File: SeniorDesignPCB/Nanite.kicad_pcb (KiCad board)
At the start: 2 copper layers, 154.9 x 76.2 mm, 20 parts, among them U1 4017, U2 TLC555

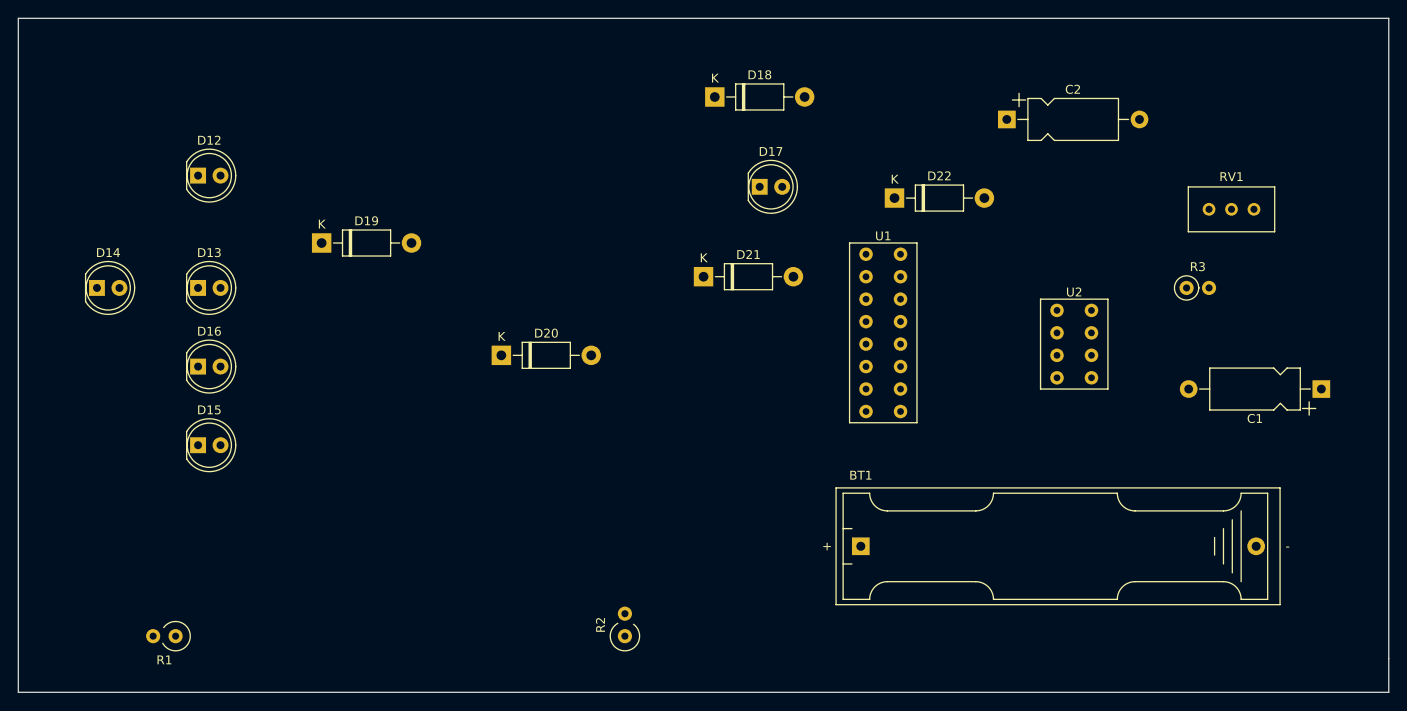
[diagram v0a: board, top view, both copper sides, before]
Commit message: Added all tracings
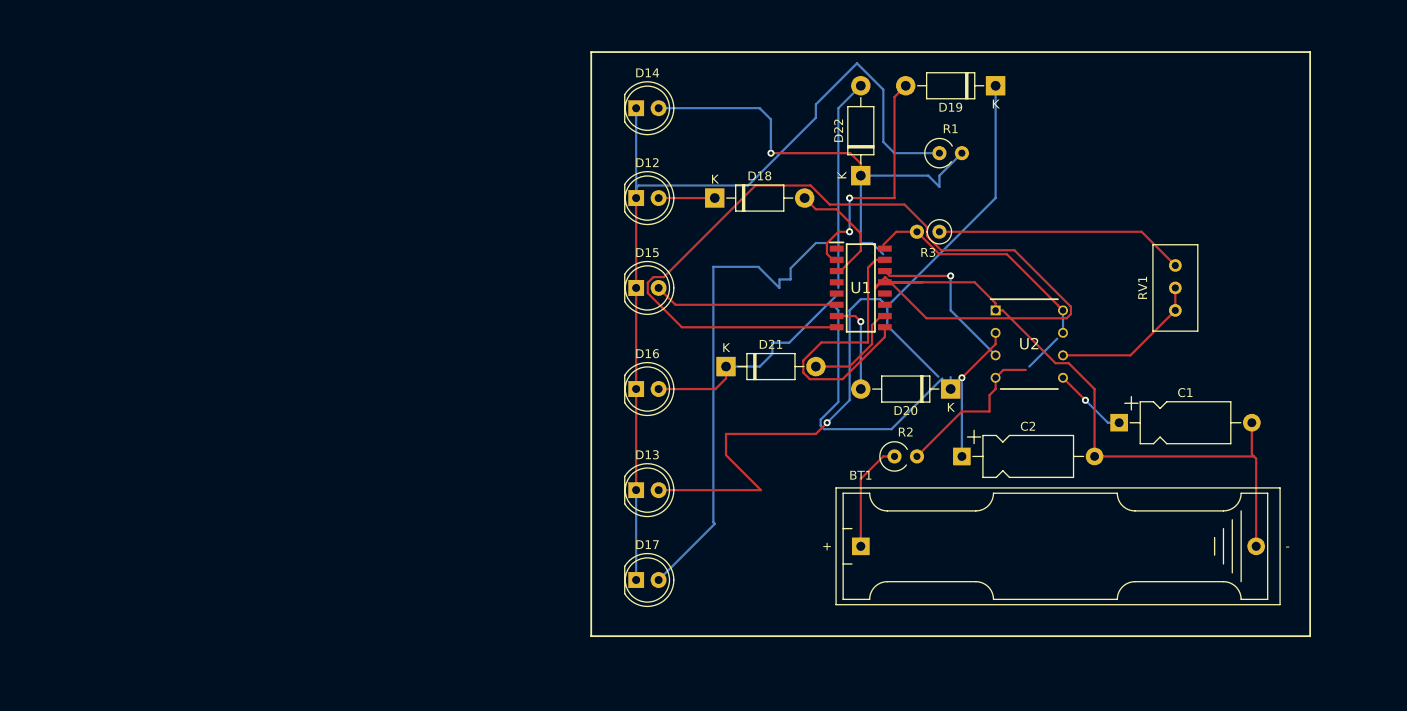
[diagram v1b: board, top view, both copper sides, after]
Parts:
- U1: footprint Johnson Counter 4017:DecadeCounter -> 74HC4017D_653:SOIC127P600X175-16N
- U2: value TLC555 -> 555TIMER; footprint 555 Timer:TLC555 -> LM555CN_Timer:DIP762W53P254L980H533Q8N
- moved R1 102.2 mm to (127.0, 77.5), turned to 0 degrees
- moved D19 78.2 mm to (133.3, 69.8), turned to 180 degrees
- moved D14 64.3 mm to (92.7, 72.4)
- moved D13 54.6 mm to (92.7, 115.6)
- moved D15 52.6 mm to (92.7, 92.7)
- moved D20 50.9 mm to (128.3, 104.1), turned to 180 degrees
- moved D12 49.6 mm to (92.7, 82.5)
- moved D16 49.6 mm to (92.7, 104.1)
- moved D17 46.6 mm to (92.7, 125.7)
- moved C2 38.4 mm to (129.5, 111.8)
- moved R2 36.6 mm to (121.9, 111.8), turned to 0 degrees
- moved R3 28.7 mm to (127.0, 86.4), turned to 180 degrees
- moved C1 23.2 mm to (147.3, 108.0), turned to 0 degrees
- moved D18 11.4 mm to (101.6, 82.5)
- moved RV1 10.9 mm to (153.7, 90.2), turned to 90 degrees
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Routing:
- net GNDA: track 0.00 -> 186.4 mm
- net Net-(D12-Pad1): track 0.00 -> 103.2 mm
- net Net-(D13-Pad2): track 0.00 -> 90.8 mm, vias 0 -> 1
- net Net-(D14-Pad2): track 0.00 -> 86.9 mm, vias 0 -> 1
- net Net-(D17-Pad2): track 0.00 -> 55.8 mm
- net Net-(D15-Pad2): track 0.00 -> 53.3 mm
- net Net-(R2-Pad2): track 0.00 -> 45.4 mm
- net Net-(R3-Pad1): track 0.00 -> 28.2 mm
- net Net-(D19-Pad2): track 0.00 -> 27.8 mm, vias 0 -> 2
- net Net-(D16-Pad2): track 0.00 -> 26.6 mm
- net Net-(D22-Pad2): track 0.00 -> 23.9 mm
- net Net-(U1-Pad14): track 0.00 -> 18.7 mm, vias 0 -> 1
- net Net-(RV1-Pad2): track 0.00 -> 17.3 mm
- net Net-(C2-Pad1): track 0.00 -> 15.5 mm, vias 0 -> 1
- net Net-(D18-Pad2): track 0.00 -> 14.1 mm
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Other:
- board outline removed
